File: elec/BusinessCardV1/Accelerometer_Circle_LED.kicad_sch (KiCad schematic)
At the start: 21 parts, among them U10 SN74LVC08APWR, U11 SN74LVC08APWR, U8 SN74LVC08APWR, U9 SN74LVC08APWR

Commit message: All footprint and start of PCB
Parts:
- D1, D10, D11, D12, D13, D14, D15, D16, D2, D3, D4, D5, D6, D7, D8, D9: footprint FP-QBLP595-R-MFG -> LED_SMD:LED_0402_1005Metric_Pad0.77x0.64mm_HandSolder
- R4: footprint (none) -> Resistor_SMD:R_0603_1608Metric_Pad0.98x0.95mm_HandSolder
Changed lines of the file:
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@@
 			)
 		)
-		(property "Footprint" "FP-QBLP595-R-MFG"
+		(property "Footprint" "LED_SMD:LED_0402_1005Metric_Pad0.77x0.64mm_HandSolder"
 			(at 110.49 105.41 0)
 			(effects
@@
 			)
 		)
-		(property "Footprint" "FP-QBLP595-R-MFG"
+		(property "Footprint" "LED_SMD:LED_0402_1005Metric_Pad0.77x0.64mm_HandSolder"
 			(at 109.22 102.87 0)
 			(effects
@@
 			)
 		)
-		(property "Footprint" "FP-QBLP595-R-MFG"
+		(property "Footprint" "LED_SMD:LED_0402_1005Metric_Pad0.77x0.64mm_HandSolder"
 			(at 167.64 55.88 0)
 			(effects
@@
 			)
 		)
-		(property "Footprint" "FP-QBLP595-R-MFG"
+		(property "Footprint" "LED_SMD:LED_0402_1005Metric_Pad0.77x0.64mm_HandSolder"
 			(at 109.22 53.34 0)
 			(effects
@@
 			)
 		)
-		(property "Footprint" "FP-QBLP595-R-MFG"
+		(property "Footprint" "LED_SMD:LED_0402_1005Metric_Pad0.77x0.64mm_HandSolder"
 			(at 167.64 58.42 0)
 			(effects
@@
 			)
 		)
-		(property "Footprint" "FP-QBLP595-R-MFG"
+		(property "Footprint" "LED_SMD:LED_0402_1005Metric_Pad0.77x0.64mm_HandSolder"
 			(at 109.22 60.96 0)
 			(effects
@@
 			)
 		)
-		(property "Footprint" ""
+		(property "Footprint" "Resistor_SMD:R_0603_1608Metric_Pad0.98x0.95mm_HandSolder"
 			(at 106.68 141.478 90)
 			(effects
@@
 			)
 		)
-		(property "Footprint" "FP-QBLP595-R-MFG"
+		(property "Footprint" "LED_SMD:LED_0402_1005Metric_Pad0.77x0.64mm_HandSolder"
 			(at 167.64 100.33 0)
 			(effects
@@
 			)
 		)
-		(property "Footprint" "FP-QBLP595-R-MFG"
+		(property "Footprint" "LED_SMD:LED_0402_1005Metric_Pad0.77x0.64mm_HandSolder"
 			(at 167.64 60.96 0)
 			(effects
@@
 			)
 		)
-		(property "Footprint" "FP-QBLP595-R-MFG"
+		(property "Footprint" "LED_SMD:LED_0402_1005Metric_Pad0.77x0.64mm_HandSolder"
 			(at 167.64 105.41 0)
 			(effects
@@
 			)
 		)
-		(property "Footprint" "FP-QBLP595-R-MFG"
+		(property "Footprint" "LED_SMD:LED_0402_1005Metric_Pad0.77x0.64mm_HandSolder"
 			(at 109.22 100.33 0)
 			(effects
@@
 			)
 		)
-		(property "Footprint" "FP-QBLP595-R-MFG"
+		(property "Footprint" "LED_SMD:LED_0402_1005Metric_Pad0.77x0.64mm_HandSolder"
 			(at 167.64 97.79 0)
 			(effects
@@
 			)
 		)
-		(property "Footprint" "FP-QBLP595-R-MFG"
+		(property "Footprint" "LED_SMD:LED_0402_1005Metric_Pad0.77x0.64mm_HandSolder"
 			(at 109.22 55.88 0)
 			(effects
@@
 			)
 		)
-		(property "Footprint" "FP-QBLP595-R-MFG"
+		(property "Footprint" "LED_SMD:LED_0402_1005Metric_Pad0.77x0.64mm_HandSolder"
 			(at 109.22 97.79 0)
 			(effects
@@
 			)
 		)
-		(property "Footprint" "FP-QBLP595-R-MFG"
+		(property "Footprint" "LED_SMD:LED_0402_1005Metric_Pad0.77x0.64mm_HandSolder"
 			(at 167.64 53.34 0)
 			(effects
@@
 			)
 		)
-		(property "Footprint" "FP-QBLP595-R-MFG"
+		(property "Footprint" "LED_SMD:LED_0402_1005Metric_Pad0.77x0.64mm_HandSolder"
 			(at 167.64 102.87 0)
 			(effects
@@
 			)
 		)
-		(property "Footprint" "FP-QBLP595-R-MFG"
+		(property "Footprint" "LED_SMD:LED_0402_1005Metric_Pad0.77x0.64mm_HandSolder"
 			(at 109.22 58.42 0)
 			(effects

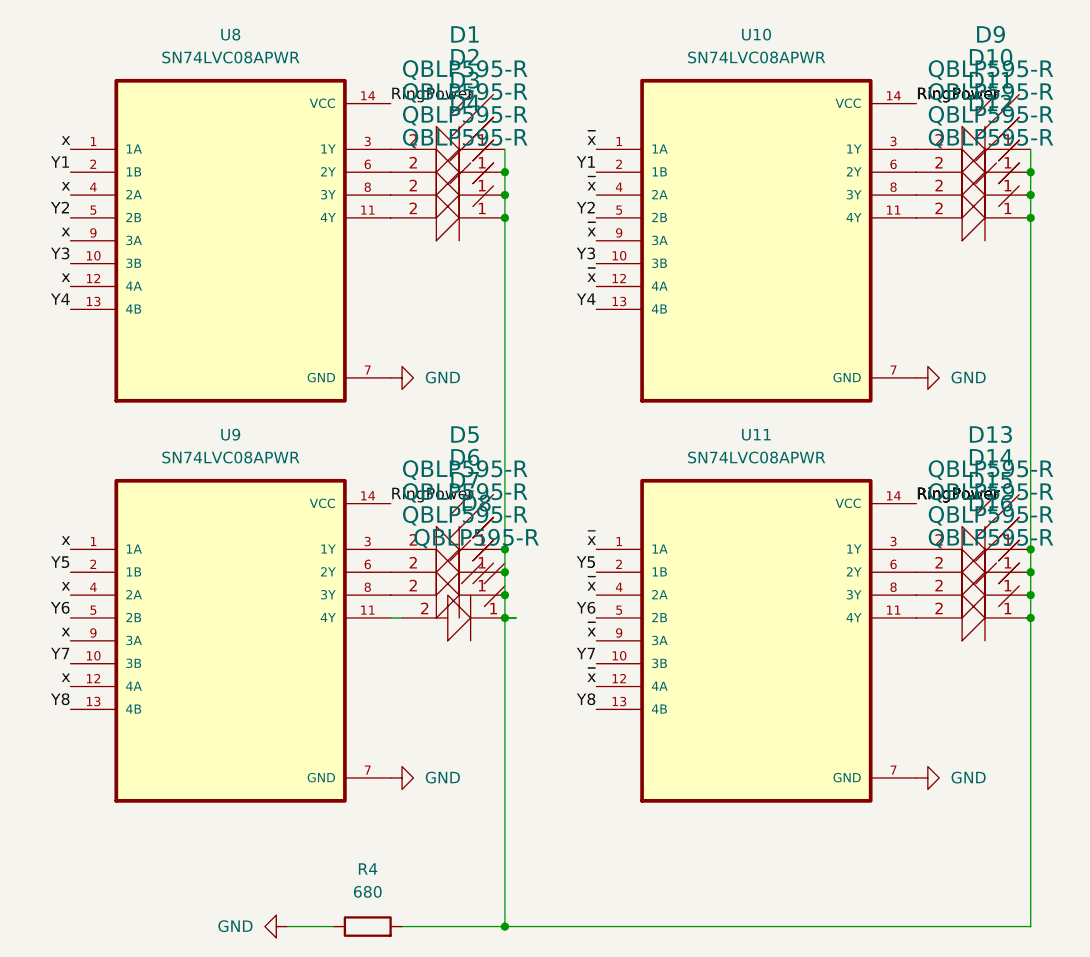
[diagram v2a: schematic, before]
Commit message: Easy part done, Glabel kind of worked
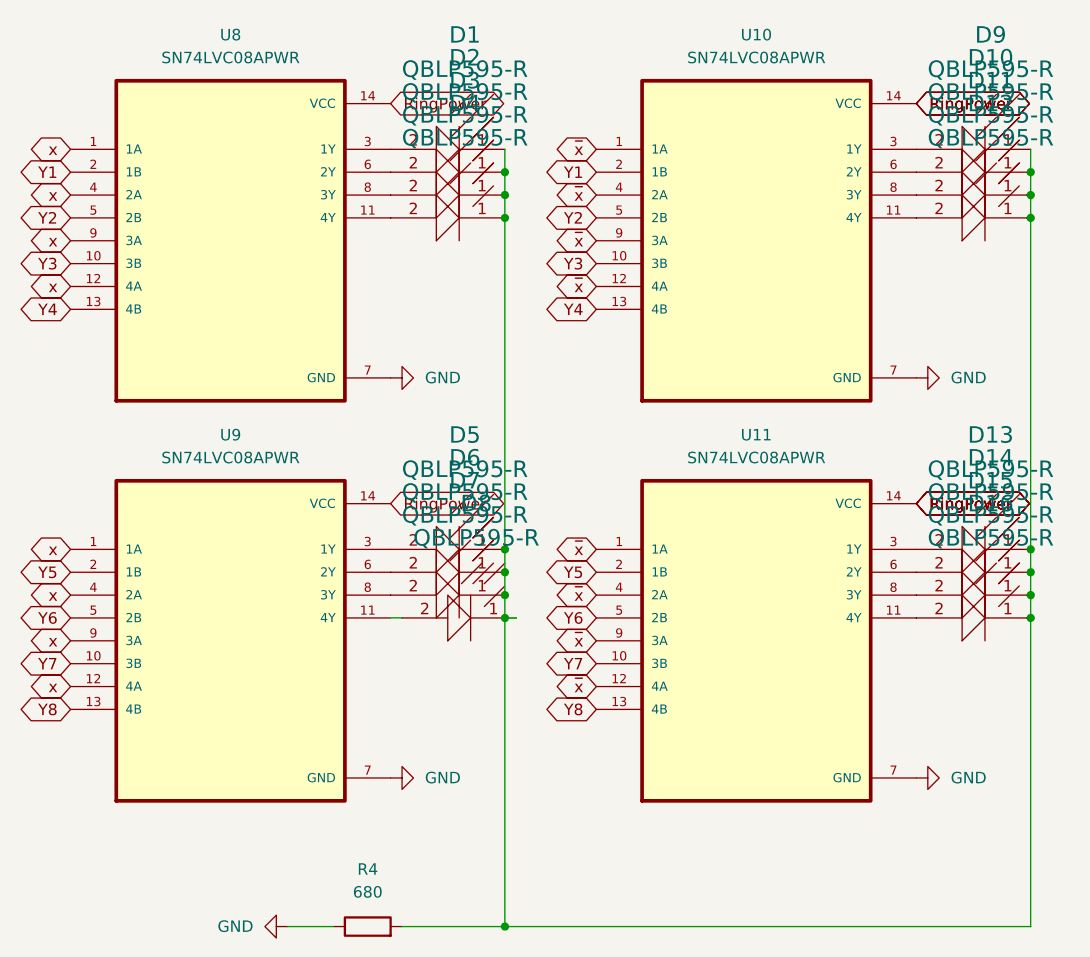
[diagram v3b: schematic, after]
